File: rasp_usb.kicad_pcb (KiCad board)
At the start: 2 copper layers, 24 x 22 mm, 23 parts, among them J1 USB_B_Micro, J2 Conn_02x05_Odd_Even, U1 AMS1117-5.0, U3 CP2104

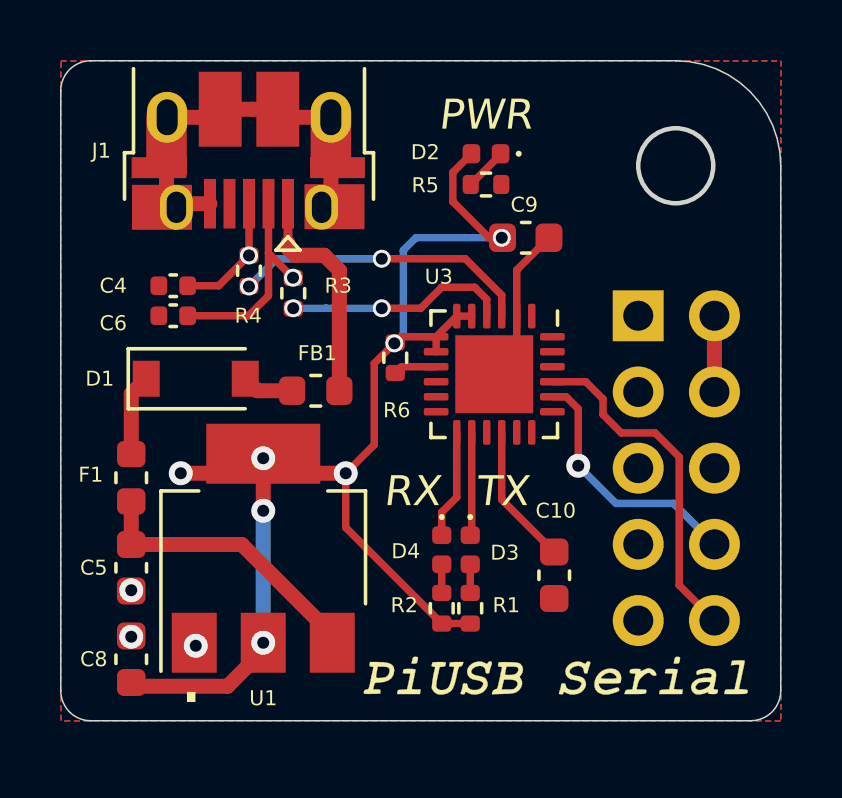
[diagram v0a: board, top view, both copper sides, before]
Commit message: ready to order
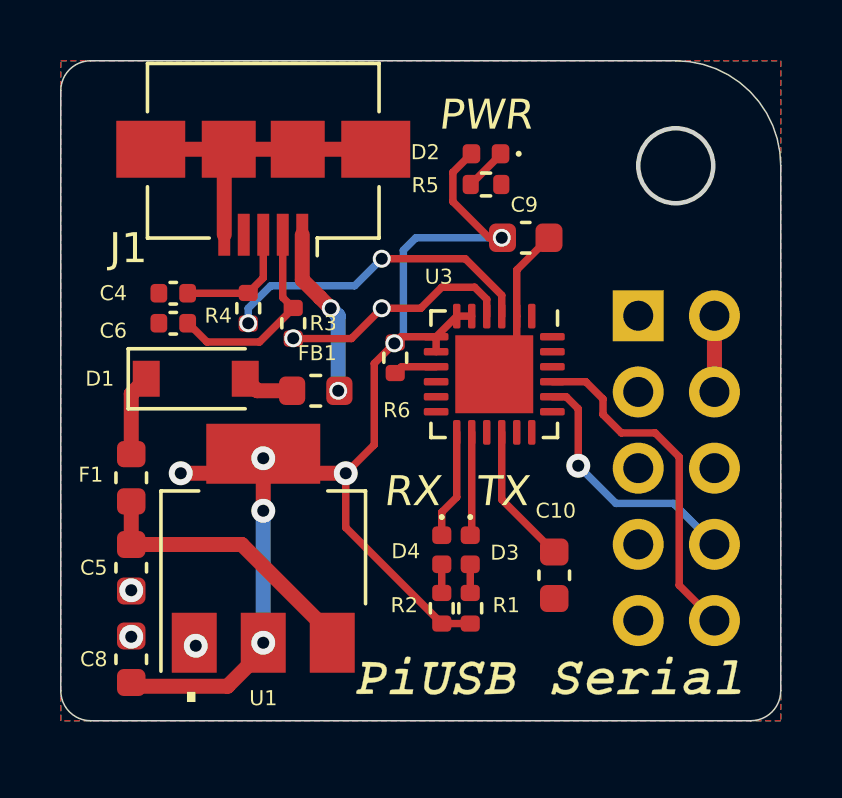
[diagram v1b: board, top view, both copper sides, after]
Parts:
- J1: footprint Connector_USB:USB_Micro-B_Amphenol_10103594-0001LF_Horizontal -> Connector_USB:USB_Micro-B_Amphenol_10104110_Horizontal
- moved J1 1.35 mm to (107.8, 64.2)
- moved R4 1.25 mm to (107.2, 68.2)
- moved R3 1.00 mm to (108.8, 68.8)
- moved C4 0.25 mm to (104.8, 67.8)
- moved C6 0.25 mm to (104.8, 68.8)
- moved G*** 0.25 mm to (117.2, 80.5)
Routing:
- net VBUS: track 7.52 -> 5.70 mm, vias 0 -> 2
- net GND: track 17.3 -> 15.7 mm
- net Net-(R4-Pad2): track 10.0 -> 10.8 mm
- net USB_DM: track 7.20 -> 6.84 mm, vias 1 -> 0
- net USB_DP: track 4.19 -> 4.17 mm, vias 1 -> 0
